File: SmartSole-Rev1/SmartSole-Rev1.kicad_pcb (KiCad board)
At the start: 2 copper layers, 38.1 x 68.6 mm, 41 parts, among them J1 5103310-5, J2 1-825433-2, J3 1-825433-2, U1 MCP6004, U2 MCP6004, U3 AD1583

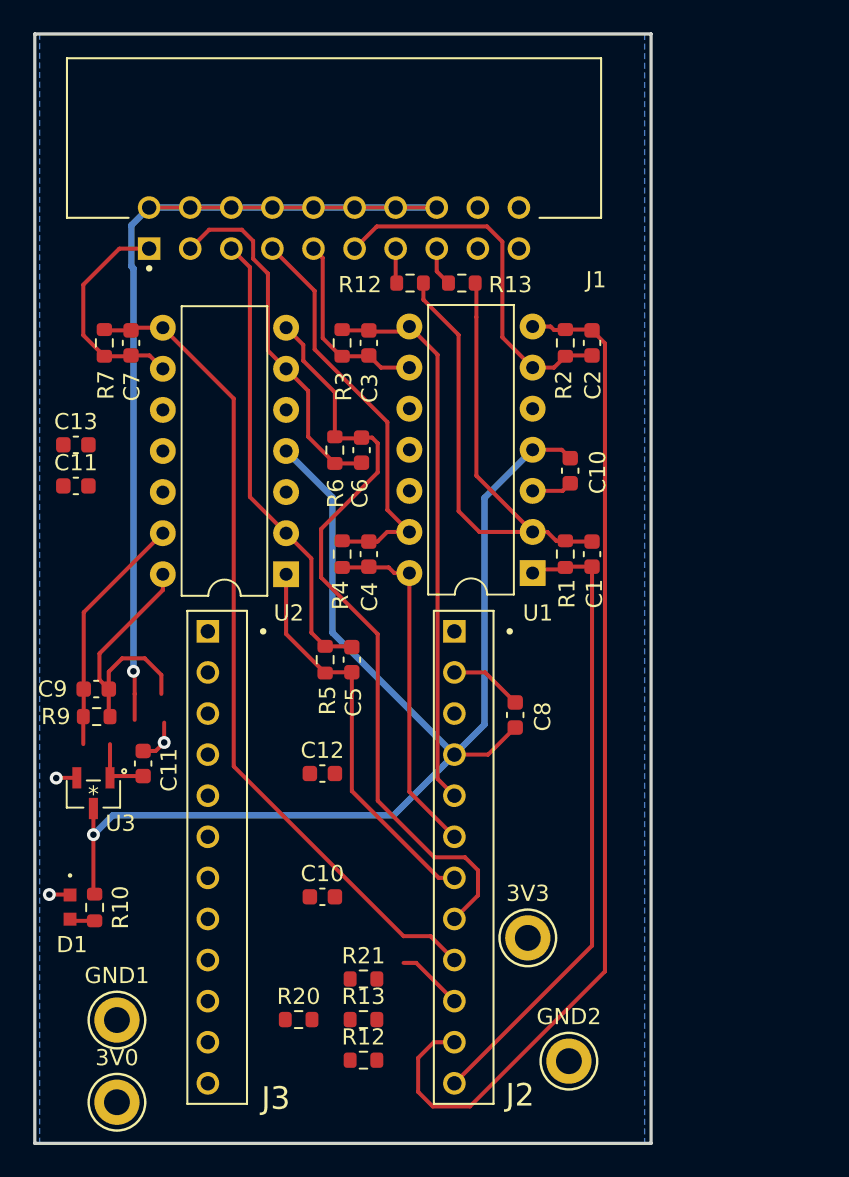
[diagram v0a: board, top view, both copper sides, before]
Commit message: final layout
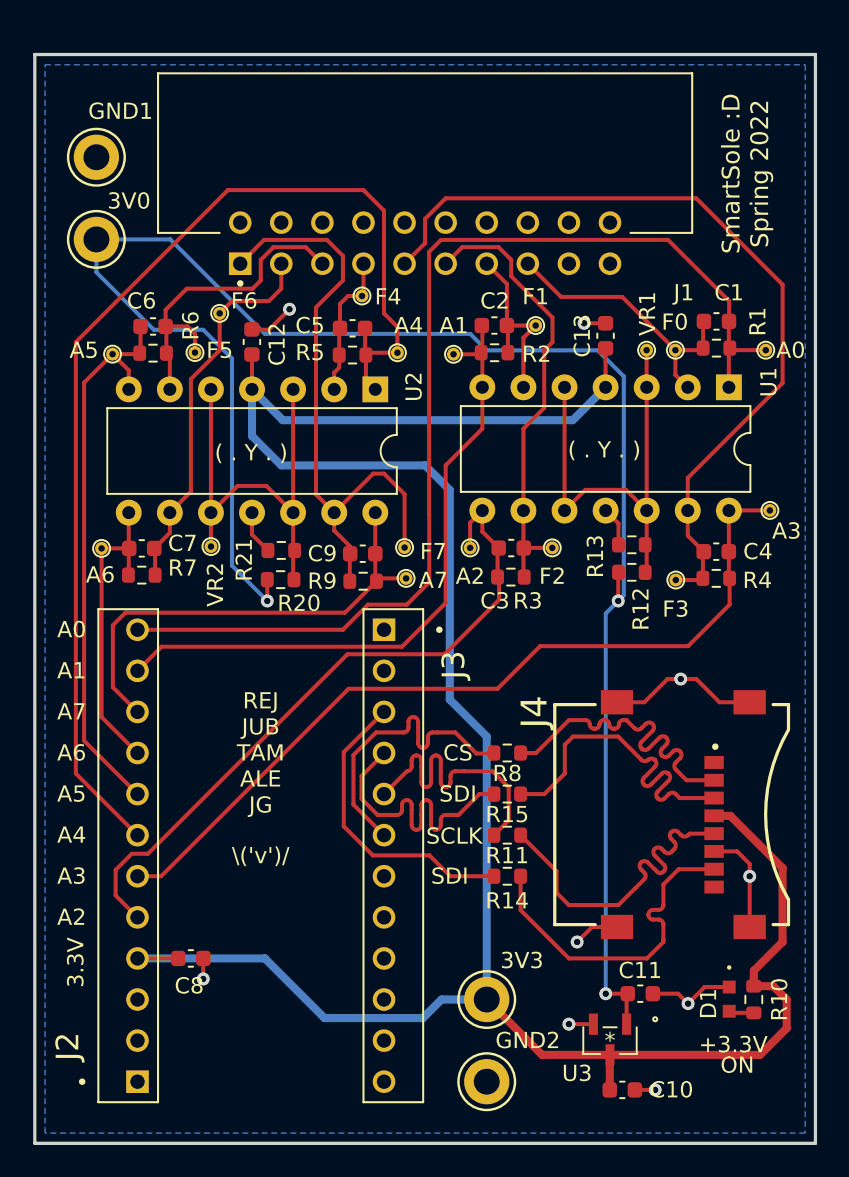
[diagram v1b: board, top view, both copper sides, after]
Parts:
- removed the C10 at (77.3, 84.7)
- removed the C11 at (66.3, 76.4)
- removed the R12 at (82.8, 46.7)
- removed the R13 at (79.9, 92.2)
- added A0: TestPoint_Small, SmartSoleFPs:TestPoint_Loop_D0.8mm_Dril0.4mm, F.Cu at (104.8, 50.9)
- added A1: TestPoint_Small, SmartSoleFPs:TestPoint_Loop_D0.8mm_Dril0.4mm, F.Cu at (85.4, 51.1)
- added A2: TestPoint_Small, SmartSoleFPs:TestPoint_Loop_D0.8mm_Dril0.4mm, F.Cu at (86.5, 63.1)
- added A3: TestPoint_Small, SmartSoleFPs:TestPoint_Loop_D0.8mm_Dril0.4mm, F.Cu at (105.0, 60.8)
- added A4: TestPoint_Small, SmartSoleFPs:TestPoint_Loop_D0.8mm_Dril0.4mm, F.Cu at (82.0, 51.0)
- added A5: TestPoint_Small, SmartSoleFPs:TestPoint_Loop_D0.8mm_Dril0.4mm, F.Cu at (64.4, 51.1)
- added A6: TestPoint_Small, SmartSoleFPs:TestPoint_Loop_D0.8mm_Dril0.4mm, F.Cu at (63.7, 63.1)
- added A7: TestPoint_Small, SmartSoleFPs:TestPoint_Loop_D0.8mm_Dril0.4mm, F.Cu at (82.5, 65.0)
- added F0: TestPoint_Small, SmartSoleFPs:TestPoint_Loop_D0.8mm_Dril0.4mm, F.Cu at (99.2, 50.9)
- added F1: TestPoint_Small, SmartSoleFPs:TestPoint_Loop_D0.8mm_Dril0.4mm, F.Cu at (90.5, 49.3)
- added F2: TestPoint_Small, SmartSoleFPs:TestPoint_Loop_D0.8mm_Dril0.4mm, F.Cu at (91.6, 63.1)
- added F3: TestPoint_Small, SmartSoleFPs:TestPoint_Loop_D0.8mm_Dril0.4mm, F.Cu at (99.2, 65.1)
- added F4: TestPoint_Small, SmartSoleFPs:TestPoint_Loop_D0.8mm_Dril0.4mm, F.Cu at (79.8, 47.5)
- added F5: TestPoint_Small, SmartSoleFPs:TestPoint_Loop_D0.8mm_Dril0.4mm, F.Cu at (69.5, 51.0)
- added F6: TestPoint_Small, SmartSoleFPs:TestPoint_Loop_D0.8mm_Dril0.4mm, F.Cu at (71.0, 48.6)
- added F7: TestPoint_Small, SmartSoleFPs:TestPoint_Loop_D0.8mm_Dril0.4mm, F.Cu at (82.4, 63.1)
- added J4: MEM2067-02-180-00-A_REVB, SmartSoleFPs:GCT_MEM2067-02-180-00-A_REVB, F.Cu at (98.9, 79.6)
- added R11: 0, Resistor_SMD:R_0603_1608Metric, F.Cu at (88.8, 80.8)
- added R14: 0, Resistor_SMD:R_0603_1608Metric, F.Cu at (88.8, 83.4)
- added R15: 0, Resistor_SMD:R_0603_1608Metric, F.Cu at (88.8, 78.3)
- added R8: 0, Resistor_SMD:R_0603_1608Metric, F.Cu at (88.8, 75.8)
- added VR1: TestPoint_Small, SmartSoleFPs:TestPoint_Loop_D0.8mm_Dril0.4mm, F.Cu at (97.4, 50.9)
- added VR2: TestPoint_Small, SmartSoleFPs:TestPoint_Loop_D0.8mm_Dril0.4mm, F.Cu at (70.5, 63.0)
- D1: footprint CapstoneLibrary:VLMG1300-GS08 -> SmartSoleFPs:VLMG1300-GS08
- J1: footprint CapstoneLibrary:TE_5103310-5 -> SmartSoleFPs:TE_5103310-5
- J2, J3: footprint CapstoneLibrary:TE_1-825433-2 -> SmartSoleFPs:TE_1-825433-2
- U3: footprint CapstoneLibrary:AD1583ARTZ-Reel7 -> SmartSoleFPs:AD1583ARTZ-Reel7
- moved GND1 53.4 mm to (63.4, 38.9)
- moved 3V0 53.4 mm to (63.4, 44.0)
- moved C11 46.9 mm to (97.0, 90.7)
- moved R10 41.1 mm to (104.0, 91.0)
- moved D1 41.1 mm to (102.5, 91.0)
- moved C10 38.4 mm to (95.9, 96.6), turned to 0 degrees
- moved U3 35.4 mm to (95.1, 93.5)
- moved R12 34.4 mm to (96.5, 64.6)
- moved C13 33.4 mm to (94.8, 50.0), turned to 90 degrees
- moved R20 27.2 mm to (74.8, 65.1)
- moved C12 27.0 mm to (73.0, 50.4), turned to 90 degrees
- moved R21 27.0 mm to (74.8, 63.2), turned to 180 degrees
- moved C8 25.1 mm to (69.2, 88.5), turned to 0 degrees
- moved R4 23.2 mm to (101.7, 65.0), turned to 0 degrees
- moved C4 21.5 mm to (101.7, 63.3), turned to 180 degrees
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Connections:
- J3 pad 3: unconnected-(J3-Pad3) -> /SDO-MISO
- J3 pad 4: unconnected-(J3-Pad4) -> /SDI-MOSI
- J3 pad 5: unconnected-(J3-Pad5) -> /SCLK
- J3 pad 6: unconnected-(J3-Pad6) -> /CS
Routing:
- net /VRef: track 4.18 -> 109.5 mm, vias 1 -> 3
- net +3V3: track 80.6 -> 143.7 mm, vias 1 -> 0
- net GND: track 82.6 -> 37.5 mm, vias 3 -> 9
- net /AIN4: track 24.7 -> 69.6 mm
- net /AIN6: track 51.2 -> 19.1 mm
- net /AIN3: track 21.8 -> 51.9 mm
- net /AIN0: track 39.3 -> 67.6 mm
- net /Op Amps/VRef2: track 0.00 -> 27.9 mm
- net /Op Amps/VRef1: track 2.16 -> 27.4 mm
- net /ForceIn_3: track 25.4 -> 50.7 mm
- net /ForceIn_0: track 40.9 -> 17.1 mm
- net /AIN1: track 63.9 -> 40.5 mm
- net /ForceIn_7: track 15.1 -> 38.2 mm
- net Net-(J4-Pad5): track 0.00 -> 21.0 mm
- net Net-(J4-Pad7): track 0.00 -> 21.0 mm
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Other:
- board size 38.1 x 68.6 mm -> 48.3 x 67.3 mm
- board text added: "( . Y . )"
- board text added: "+3.3V"
- board text added: "0 mm"
- board text added: "0.01 mm"
- board text added: "0.035 mm"
- board text added: "0.1524 mm / 0.1524 mm"
- board text added: "0.3000 mm"
- board text added: "1.51 mm"
- board text added: "1.6000 mm"
- board text added: "3.3V"
- board text added: "48.4600 mm x 67.5100 mm"
- board text added: "A0"
- board text added: "A1"
- board text added: "A2"
- board text added: "A3"
- board text added: "A4"
- board text added: "A5"
- board text added: "A6"
- board text added: "A7"
- board text added: "CS"
- board text added: "Dielectric"
- board text added: "ON"
- board text added: "REJ JUB TAM ALE JG"
- board text added: "SCLK"
- board text added: "SDI"
- board text added: "SmartSole :D Spring 2022"
- board text added: "Thickness (mm)"
- board text added: "\('v')/"
- board text removed: "0 mils"
- board text removed: "0.3937008 mils"
- board text removed: "1.377953 mils"
- board text removed: "11.81 mils"
- board text removed: "1507.87 mils x 2707.87 mils"
- board text removed: "59.44882 mils"
- board text removed: "6.00 mils / 6.00 mils"
- board text removed: "62.99 mils"
- board text removed: "Dielectric 1"
- board text removed: "Thickness (mils)"
